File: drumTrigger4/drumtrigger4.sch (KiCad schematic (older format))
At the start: 24 parts, among them J1 Input, J2 TrigOut, J3 CVout, J4 Power, J5 Gain, U1 TL074

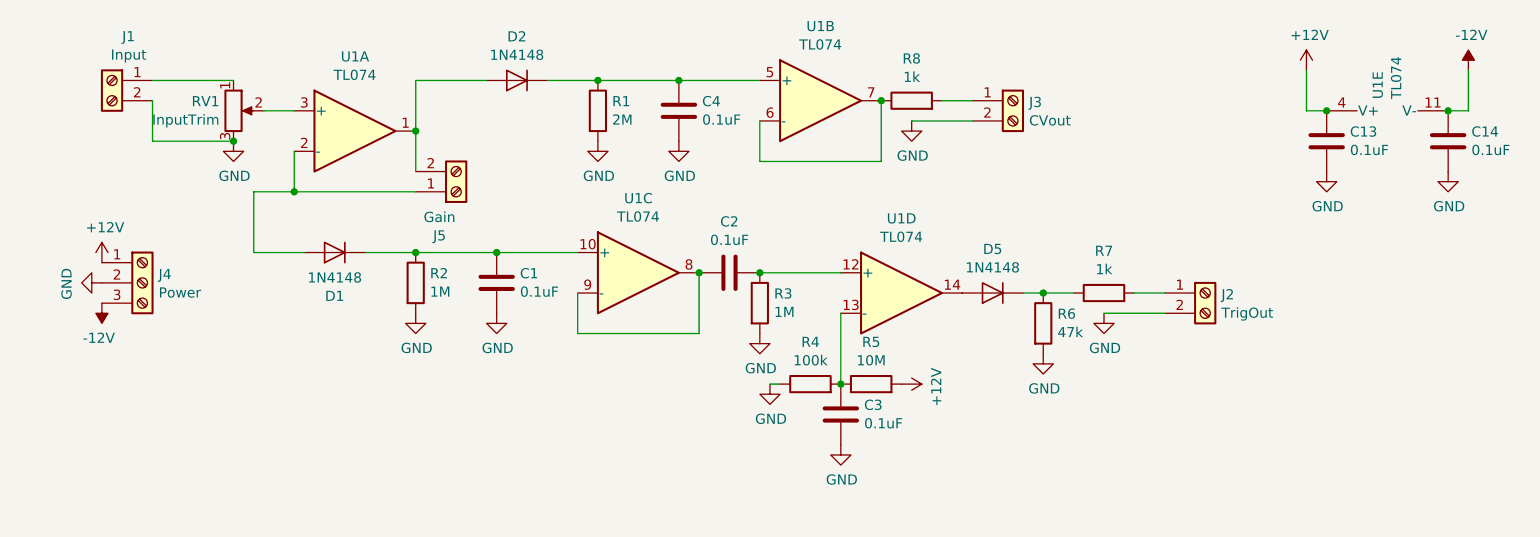
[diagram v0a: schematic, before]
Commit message: printed
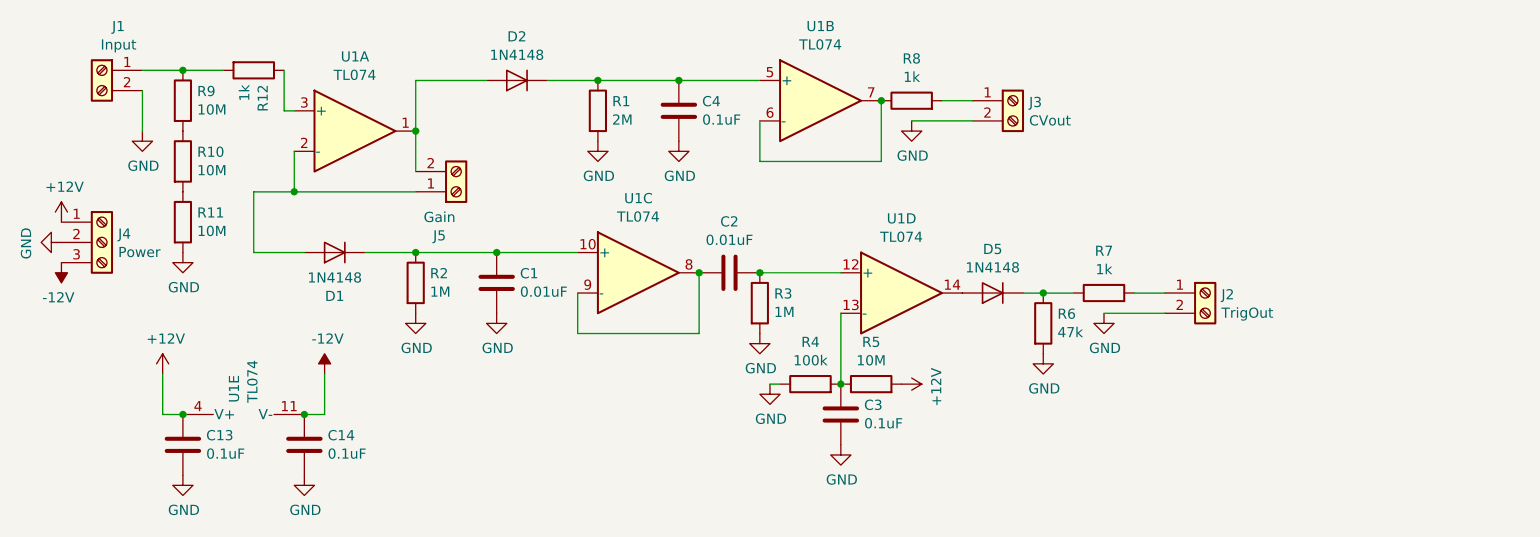
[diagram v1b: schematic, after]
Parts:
- removed RV1: InputTrim, Potentiometer_THT:Potentiometer_Piher_PT-6-V_Vertical, symbol Device:R_POT
- added R10, R11, R9: 10M, Resistor_THT:R_Axial_DIN0207_L6.3mm_D2.5mm_P10.16mm_Horizontal, symbol Device:R
- added R12: 1k, Resistor_THT:R_Axial_DIN0207_L6.3mm_D2.5mm_P10.16mm_Horizontal, symbol Device:R
- C1, C2: value 0.1uF -> 0.01uF
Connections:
- net GND: now also R11.2
- net at J1.1 (Pin_1): now also R12.2, R9.1
- net at U1.3 (+): now also R12.1
- new net: R10.1, R9.2
- new net: R10.2, R11.1
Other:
- moved on the sheet: C13, C14, J1, J4, U1E
